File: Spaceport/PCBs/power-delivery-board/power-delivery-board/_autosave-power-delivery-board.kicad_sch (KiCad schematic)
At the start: 26 parts, among them J1 Conn_01x03_Pin, U1 ADP5033ACBZ-5-R7, U2 TPS610986DSER, U3 TPS610986DSER

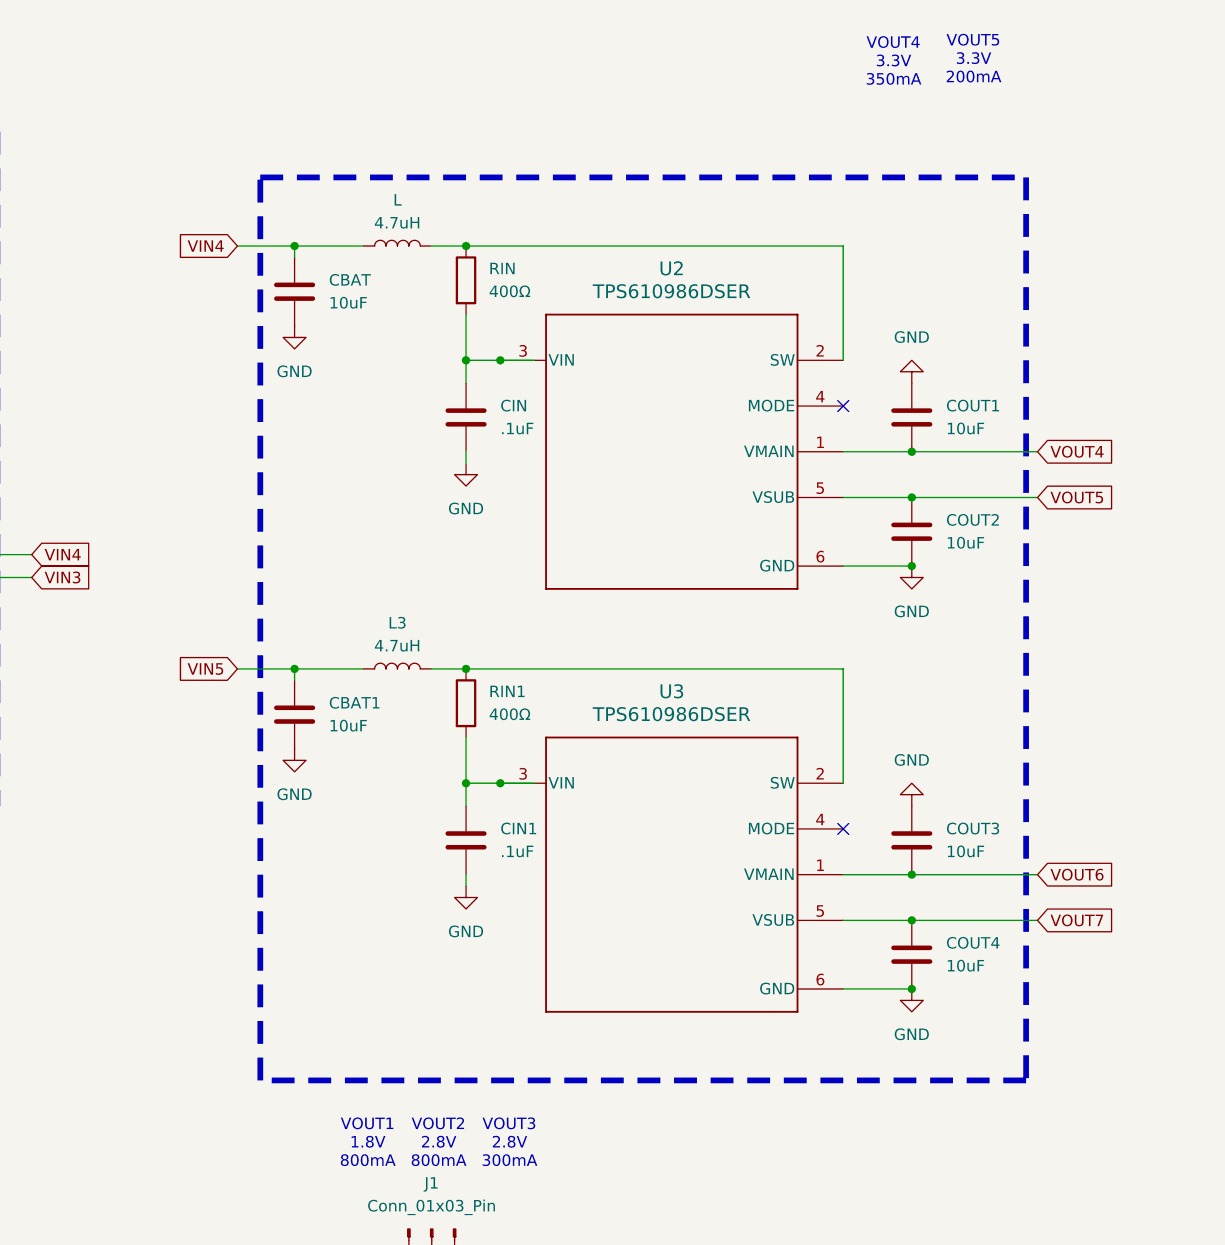
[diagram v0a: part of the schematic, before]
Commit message: Added Second Switching Regulator
Source 2 and 3:
https://www.ti.com/lit/ds/symlink/tps610985.pdf?HQS=dis-dk-null-digikeymode-dsf-pf-null-wwe&ts=1731884554797&ref_url=https%253A%252F%252Fwww.ti.com%252Fgeneral%252Fdocs%252Fsuppproductinfo.tsp%253FdistId%253D10%2526gotoUrl%253Dhttps%253A%252F%252Fwww.ti.com%252Flit%252Fgpn%252Ftps610985
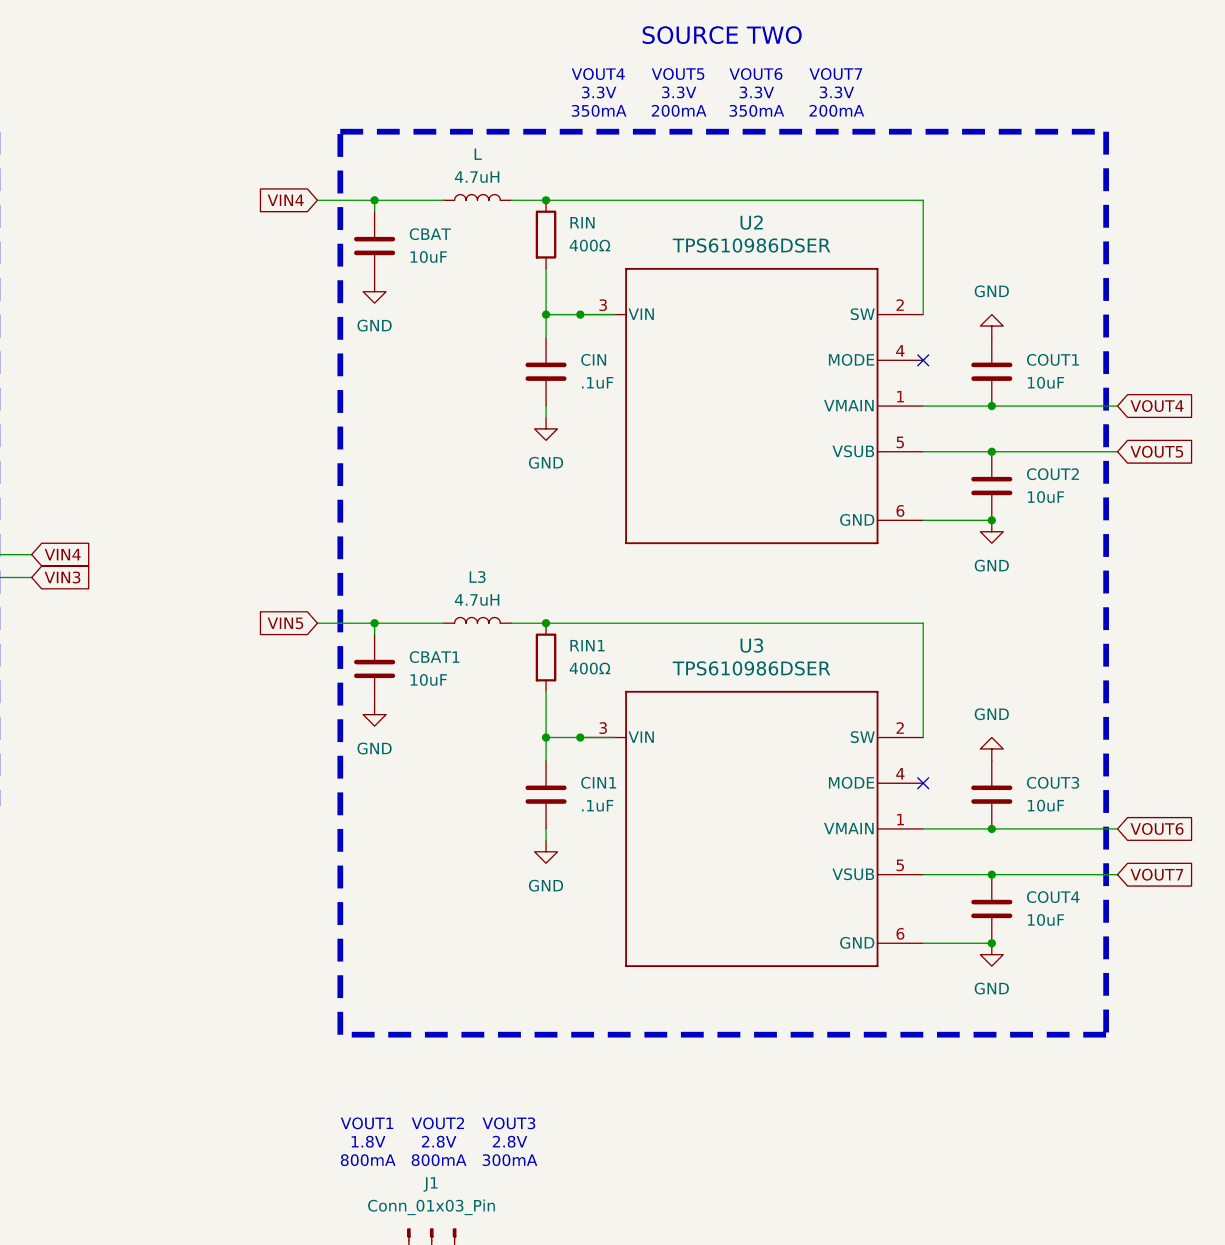
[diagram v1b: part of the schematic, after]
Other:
- note added: "SOURCE TWO"
- note added: "VOUT6 3.3V 350mA"
- note added: "VOUT7 3.3V 200mA"
- moved on the sheet: CBAT, CBAT1, CIN, CIN1, COUT1, COUT2, COUT3, COUT4, L, L3, RIN, RIN1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
